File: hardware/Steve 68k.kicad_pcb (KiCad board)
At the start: 2 copper layers, 99 x 98.9 mm, 43 parts, among them IC1 MC68008FN8, J1 Power, J2 I2C, J3 Debug, J4 ICSP, J5 Serial 1, SW1 Reset, U1 74HC04, U2 74HC32, U3 74HC138, U4 74HC257, U5 AS6C4008-55PCN, U6 28C256, U7 ATmega1284P-P, U8 Max705, X1 8Mhz

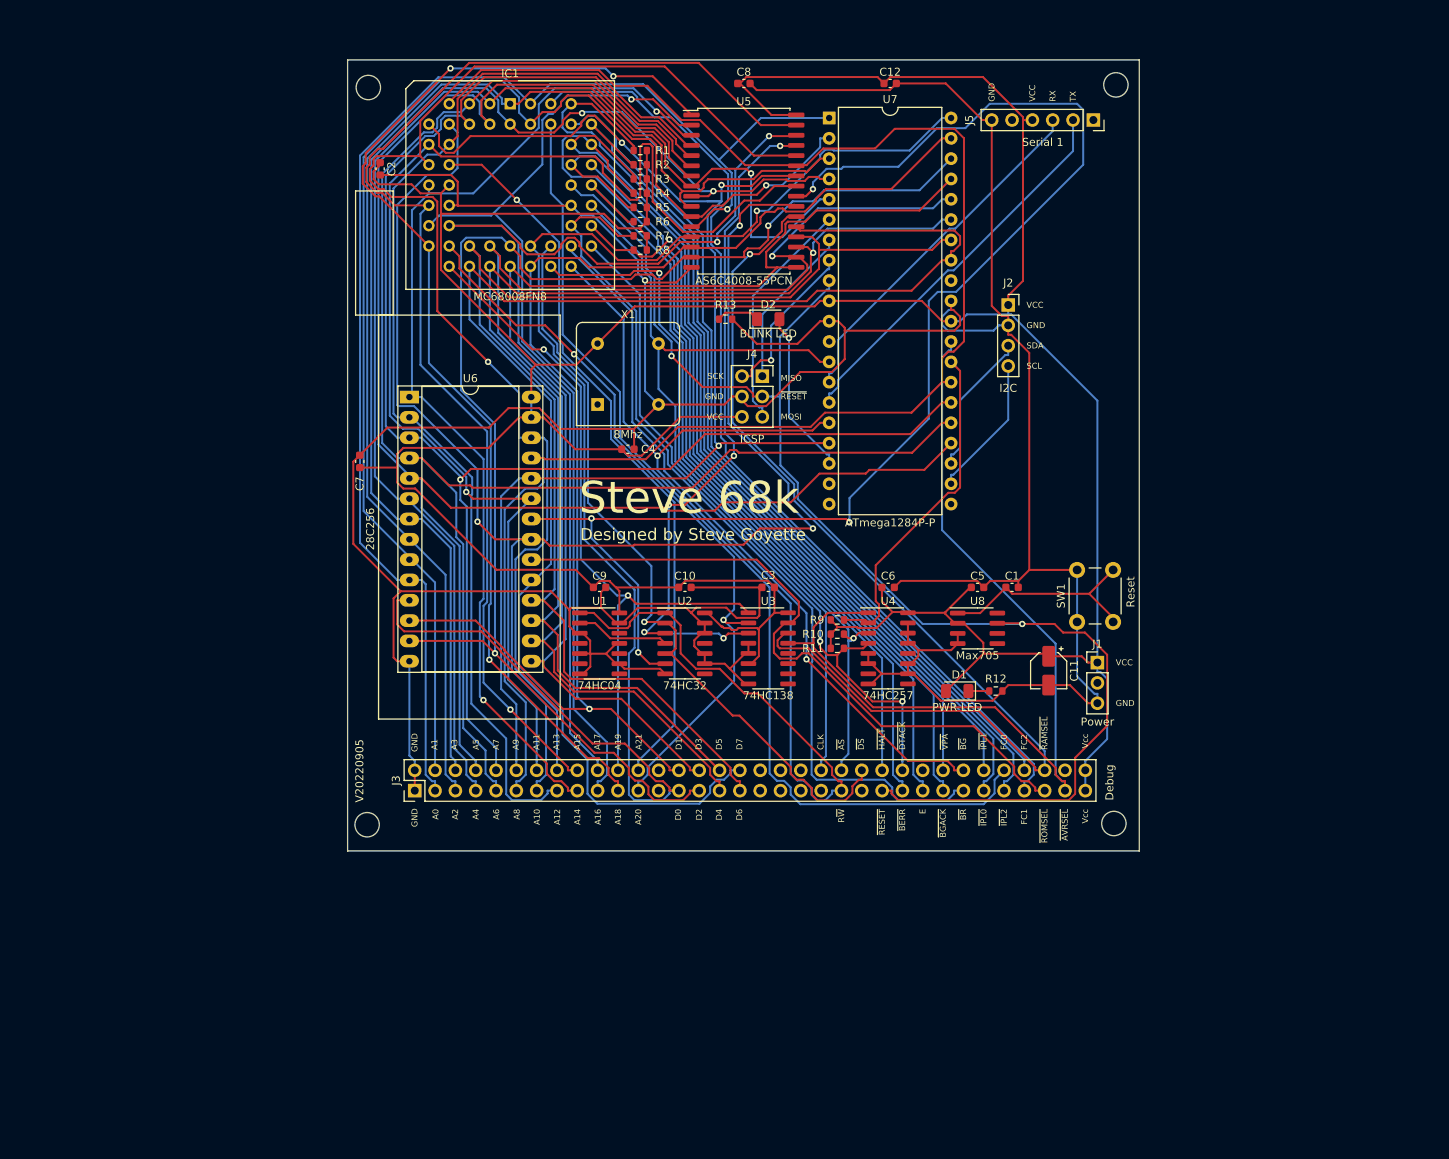
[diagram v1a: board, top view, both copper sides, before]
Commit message: V20221121
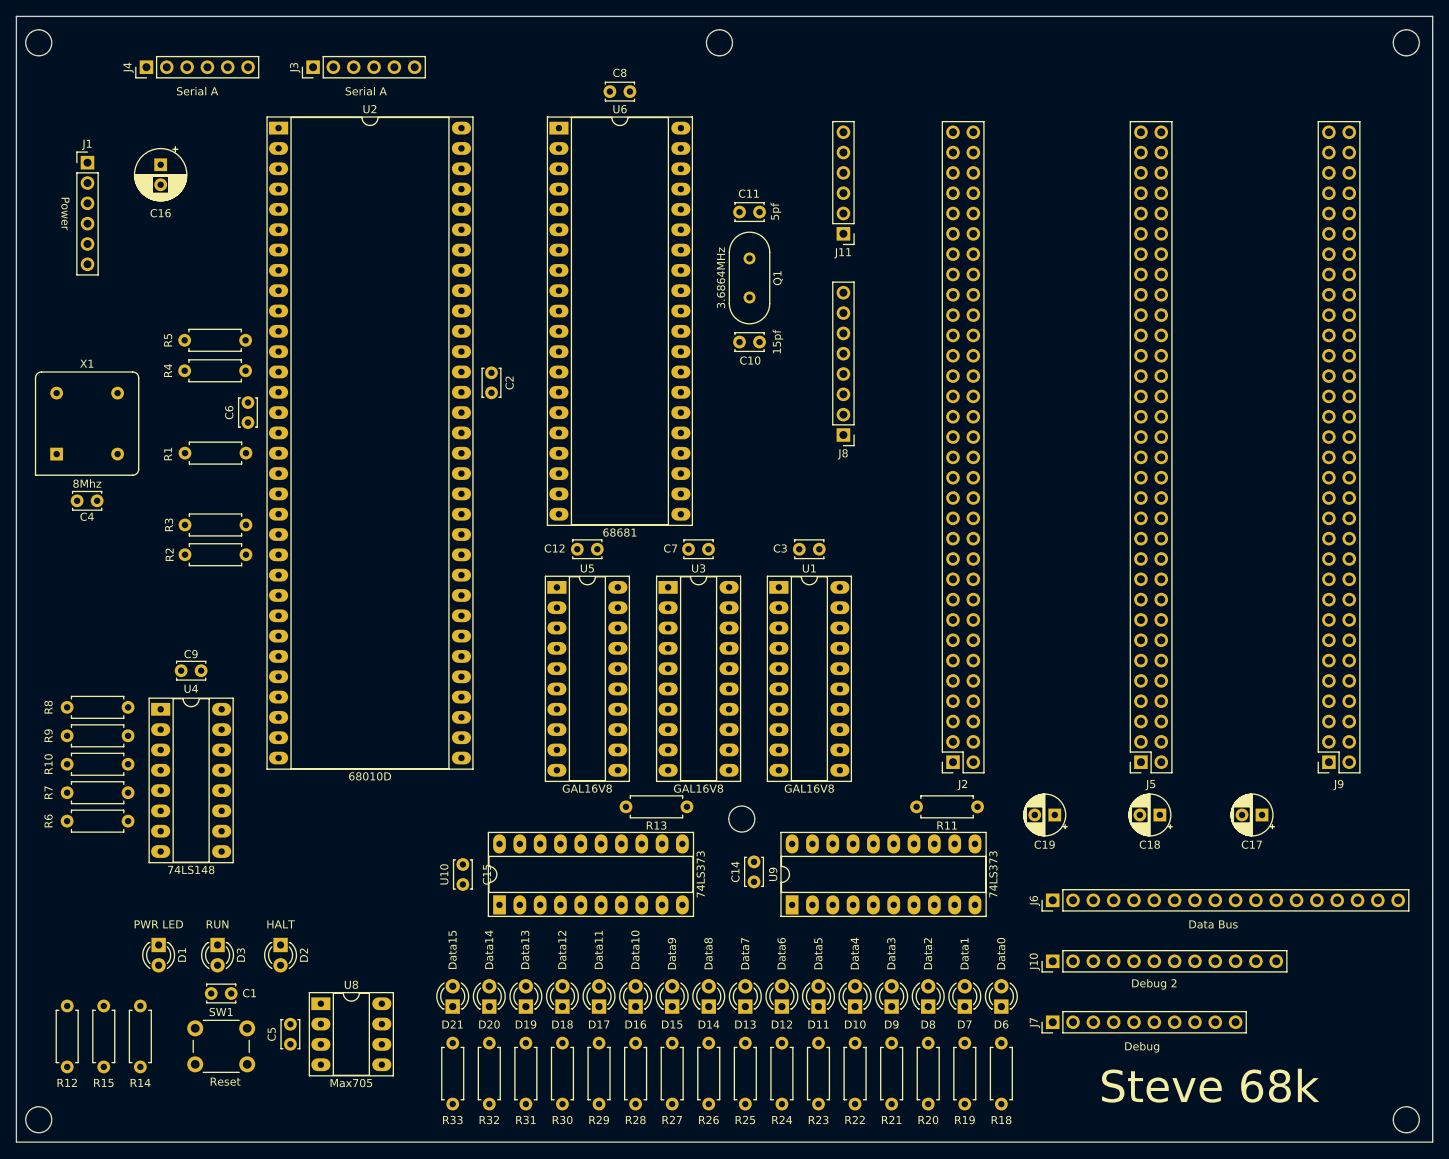
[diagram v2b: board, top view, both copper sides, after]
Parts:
- removed IC1: MC68008FN8, Package_LCC:PLCC-52_THT-Socket
- removed U7: ATmega1284P-P, Package_DIP:DIP-40_W15.24mm
- added C14: .1uF, Capacitor_THT:C_Disc_D3.4mm_W2.1mm_P2.50mm, F.Cu at (114.6, 136.7)
- added C15: .1uF, Capacitor_THT:C_Disc_D3.4mm_W2.1mm_P2.50mm, F.Cu at (78.2, 137.0)
- added C16: 470uF, Capacitor_THT:CP_Radial_D6.3mm_P2.50mm, F.Cu at (40.4, 49.5)
- added C17: 100uF, Capacitor_THT:CP_Radial_D5.0mm_P2.50mm, F.Cu at (178.1, 130.8)
- added C18: 100uF, Capacitor_THT:CP_Radial_D5.0mm_P2.50mm, F.Cu at (165.3, 130.8)
- added C19: 100uF, Capacitor_THT:CP_Radial_D5.0mm_P2.50mm, F.Cu at (152.1, 130.8)
- added D10: Data4, LED_THT:LED_D3.0mm_Clear, F.Cu at (127.2, 154.8)
- added D11: Data5, LED_THT:LED_D3.0mm_Clear, F.Cu at (122.6, 154.8)
- added D12: Data6, LED_THT:LED_D3.0mm_Clear, F.Cu at (118.0, 154.8)
- added D13: Data7, LED_THT:LED_D3.0mm_Clear, F.Cu at (113.5, 154.8)
- added D14: Data8, LED_THT:LED_D3.0mm_Clear, F.Cu at (108.9, 154.8)
- added D15: Data9, LED_THT:LED_D3.0mm_Clear, F.Cu at (104.3, 154.8)
- added D16: Data10, LED_THT:LED_D3.0mm_Clear, F.Cu at (99.8, 154.8)
- added D17: Data11, LED_THT:LED_D3.0mm_Clear, F.Cu at (95.2, 154.8)
- added D18: Data12, LED_THT:LED_D3.0mm_Clear, F.Cu at (90.6, 154.8)
- added D19: Data13, LED_THT:LED_D3.0mm_Clear, F.Cu at (86.0, 154.8)
- added D20: Data14, LED_THT:LED_D3.0mm_Clear, F.Cu at (81.5, 154.8)
- added D21: Data15, LED_THT:LED_D3.0mm_Clear, F.Cu at (76.9, 154.8)
- added D3: RUN, LED_THT:LED_D3.0mm_Clear, F.Cu at (47.5, 147.1)
- added D6: Data0, LED_THT:LED_D3.0mm_Clear, F.Cu at (145.5, 154.8)
- added D7: Data1, LED_THT:LED_D3.0mm_Clear, F.Cu at (140.9, 154.8)
- added D8: Data2, LED_THT:LED_D3.0mm_Clear, F.Cu at (136.3, 154.8)
- added D9: Data3, LED_THT:LED_D3.0mm_Clear, F.Cu at (131.8, 154.8)
- added J10: Debug 2, Connector_PinHeader_2.54mm:PinHeader_1x12_P2.54mm_Vertical, F.Cu at (151.9, 149.1)
- added J11: Duart IP, Connector_PinHeader_2.54mm:PinHeader_1x06_P2.54mm_Vertical, F.Cu at (125.7, 58.2)
- added J6: Data Bus, Connector_PinHeader_2.54mm:PinHeader_1x18_P2.54mm_Vertical, F.Cu at (151.9, 141.5)
- added J7: Debug, Connector_PinHeader_2.54mm:PinHeader_1x10_P2.54mm_Vertical, F.Cu at (151.9, 156.7)
- added J8: Duart OP, Connector_PinHeader_2.54mm:PinHeader_1x08_P2.54mm_Vertical, F.Cu at (125.7, 83.3)
- added J9: Conn_02x32_Odd_Even, Connector_PinSocket_2.54mm:PinSocket_2x32_P2.54mm_Vertical, F.Cu at (186.4, 124.2)
- added Q1: 3.6864MHz, Crystal:Crystal_HC49-4H_Vertical, F.Cu at (114.0, 61.2)
- added R14: 470, Resistor_THT:R_Axial_DIN0207_L6.3mm_D2.5mm_P7.62mm_Horizontal, F.Cu at (37.8, 162.3)
- added R15: 470, Resistor_THT:R_Axial_DIN0207_L6.3mm_D2.5mm_P7.62mm_Horizontal, F.Cu at (33.3, 162.3)
- added R18: 470, Resistor_THT:R_Axial_DIN0207_L6.3mm_D2.5mm_P7.62mm_Horizontal, F.Cu at (145.5, 166.9)
- added R19: 470, Resistor_THT:R_Axial_DIN0207_L6.3mm_D2.5mm_P7.62mm_Horizontal, F.Cu at (140.9, 166.9)
- added R20: 470, Resistor_THT:R_Axial_DIN0207_L6.3mm_D2.5mm_P7.62mm_Horizontal, F.Cu at (136.3, 166.9)
- added R21: 470, Resistor_THT:R_Axial_DIN0207_L6.3mm_D2.5mm_P7.62mm_Horizontal, F.Cu at (131.8, 166.9)
- added R22: 470, Resistor_THT:R_Axial_DIN0207_L6.3mm_D2.5mm_P7.62mm_Horizontal, F.Cu at (127.2, 166.9)
- added R23: 470, Resistor_THT:R_Axial_DIN0207_L6.3mm_D2.5mm_P7.62mm_Horizontal, F.Cu at (122.6, 166.9)
- added R24: 470, Resistor_THT:R_Axial_DIN0207_L6.3mm_D2.5mm_P7.62mm_Horizontal, F.Cu at (118.0, 166.9)
- added R25: 470, Resistor_THT:R_Axial_DIN0207_L6.3mm_D2.5mm_P7.62mm_Horizontal, F.Cu at (113.5, 166.9)
- added R26: 470, Resistor_THT:R_Axial_DIN0207_L6.3mm_D2.5mm_P7.62mm_Horizontal, F.Cu at (108.9, 166.9)
- added R27: 470, Resistor_THT:R_Axial_DIN0207_L6.3mm_D2.5mm_P7.62mm_Horizontal, F.Cu at (104.3, 166.9)
- added R28: 470, Resistor_THT:R_Axial_DIN0207_L6.3mm_D2.5mm_P7.62mm_Horizontal, F.Cu at (99.8, 166.9)
- added R29: 470, Resistor_THT:R_Axial_DIN0207_L6.3mm_D2.5mm_P7.62mm_Horizontal, F.Cu at (95.2, 166.9)
- added R30: 470, Resistor_THT:R_Axial_DIN0207_L6.3mm_D2.5mm_P7.62mm_Horizontal, F.Cu at (90.6, 166.9)
- added R31: 470, Resistor_THT:R_Axial_DIN0207_L6.3mm_D2.5mm_P7.62mm_Horizontal, F.Cu at (86.0, 166.9)
- added R32: 470, Resistor_THT:R_Axial_DIN0207_L6.3mm_D2.5mm_P7.62mm_Horizontal, F.Cu at (81.5, 166.9)
- added R33: 470, Resistor_THT:R_Axial_DIN0207_L6.3mm_D2.5mm_P7.62mm_Horizontal, F.Cu at (76.9, 166.9)
- added U10: 74LS373, Package_DIP:DIP-20_W7.62mm_Socket_LongPads, F.Cu at (82.7, 142.1)
- added U9: 74LS373, Package_DIP:DIP-20_W7.62mm_Socket_LongPads, F.Cu at (119.3, 142.1)
- C1, C12, C2, C3, C4, C5, C6, C7, C8, C9: footprint Capacitor_SMD:C_0603_1608Metric -> Capacitor_THT:C_Disc_D3.4mm_W2.1mm_P2.50mm
- C10: value .1uF -> 15pf; footprint Capacitor_SMD:C_0603_1608Metric -> Capacitor_THT:C_Disc_D3.4mm_W2.1mm_P2.50mm
- C11: value 100uF -> 5pf; footprint Capacitor_SMD:CP_Elec_4x5.4 -> Capacitor_THT:C_Disc_D3.4mm_W2.1mm_P2.50mm
- D1: footprint LED_SMD:LED_1206_3216Metric -> LED_THT:LED_D3.0mm_Clear
- D2: value BLINK LED -> HALT; footprint LED_SMD:LED_1206_3216Metric -> LED_THT:LED_D3.0mm_Clear
- J1: footprint Connector_PinHeader_2.54mm:PinHeader_1x03_P2.54mm_Vertical -> Connector_PinHeader_2.54mm:PinHeader_1x06_P2.54mm_Vertical
- J2: value I2C -> Conn_02x32_Odd_Even; footprint Connector_PinSocket_2.54mm:PinSocket_1x04_P2.54mm_Vertical -> Connector_PinSocket_2.54mm:PinSocket_2x32_P2.54mm_Vertical
- J3: value Debug -> Serial A; footprint Connector_PinHeader_2.54mm:PinHeader_2x34_P2.54mm_Vertical -> Connector_PinHeader_2.54mm:PinHeader_1x06_P2.54mm_Vertical
- J4: value ICSP -> Serial A; footprint Connector_PinSocket_2.54mm:PinSocket_2x03_P2.54mm_Vertical -> Connector_PinHeader_2.54mm:PinHeader_1x06_P2.54mm_Vertical
- J5: value Serial 1 -> Conn_02x32_Odd_Even; footprint Connector_PinSocket_2.54mm:PinSocket_1x06_P2.54mm_Vertical -> Connector_PinSocket_2.54mm:PinSocket_2x32_P2.54mm_Vertical
- R1: value 10k -> Rk7; footprint Resistor_SMD:R_0603_1608Metric -> Resistor_THT:R_Axial_DIN0207_L6.3mm_D2.5mm_P7.62mm_Horizontal
- R10, R2, R3, R4, R5, R6, R7, R8, R9: value 10k -> 4K7; footprint Resistor_SMD:R_0603_1608Metric -> Resistor_THT:R_Axial_DIN0207_L6.3mm_D2.5mm_P7.62mm_Horizontal
- R11: value 10k -> 4k7; footprint Resistor_SMD:R_0603_1608Metric -> Resistor_THT:R_Axial_DIN0207_L6.3mm_D2.5mm_P7.62mm_Horizontal
- R12: value 220 -> 470; footprint Resistor_SMD:R_0603_1608Metric -> Resistor_THT:R_Axial_DIN0207_L6.3mm_D2.5mm_P7.62mm_Horizontal
- R13: value 220 -> 4k7; footprint Resistor_SMD:R_0603_1608Metric -> Resistor_THT:R_Axial_DIN0207_L6.3mm_D2.5mm_P7.62mm_Horizontal
- U1: value 74HC04 -> GAL16V8; footprint Package_SO:SOIC-14_3.9x8.7mm_P1.27mm -> Package_DIP:DIP-20_W7.62mm_Socket_LongPads
- U2: value 74HC32 -> 68010D; footprint Package_SO:SOIC-14_3.9x8.7mm_P1.27mm -> Package_DIP:DIP-64_W22.86mm_Socket_LongPads
- U3: value 74HC138 -> GAL16V8; footprint Package_SO:SOIC-16_3.9x9.9mm_P1.27mm -> Package_DIP:DIP-20_W7.62mm_Socket_LongPads
- U4: value 74HC257 -> 74LS148; footprint Package_SO:SOIC-16_3.9x9.9mm_P1.27mm -> Package_DIP:DIP-16_W7.62mm_Socket_LongPads
- U5: value AS6C4008-55PCN -> GAL16V8; footprint Package_SO:SSOP-32_11.305x20.495mm_P1.27mm -> Package_DIP:DIP-20_W7.62mm_Socket_LongPads
- U6: value 28C256 -> 68681; footprint Package_DIP:DIP-28_W15.24mm_Socket_LongPads -> Package_DIP:DIP-40_W15.24mm_Socket_LongPads
- U8: footprint Package_SO:SOIC-8_3.9x4.9mm_P1.27mm -> Package_DIP:DIP-8_W7.62mm_Socket_LongPads
- moved J1 140.9 mm to (31.2, 49.3)
- moved R12 125.2 mm to (28.7, 162.3), turned to 90 degrees
- moved SW1 121.4 mm to (44.7, 157.5), turned to 0 degrees
- moved C1 110.0 mm to (49.2, 153.1), turned to 180 degrees
- moved D1 104.7 mm to (40.1, 147.1), turned to -90 degrees
- moved R6 103.7 mm to (28.7, 131.6), turned to 0 degrees
- moved C5 103.1 mm to (56.6, 159.5), turned to 90 degrees
- moved R7 99.9 mm to (28.7, 128.0), turned to 0 degrees
- moved D2 99.2 mm to (55.4, 147.1), turned to -90 degrees
- moved R10 97.6 mm to (28.7, 124.5)
- moved R9 97.4 mm to (28.7, 120.9)
- moved U8 94.5 mm to (60.4, 154.4)
- moved R8 91.6 mm to (28.7, 117.4), turned to 0 degrees
- moved J3 91.3 mm to (59.4, 37.3)
- moved U4 91.3 mm to (40.4, 117.6)
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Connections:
- C10 pad 1: VCC -> Net-(C10-Pad1)
- C11 pad 1: VCC -> Net-(C11-Pad1)
- C2 pad 1: VCC -> GND
- C2 pad 2: GND -> VCC
- C6 pad 1: VCC -> GND
- C6 pad 2: GND -> VCC
- D1 pad 1: Net-(D1-Pad1) -> VCC
- D1 pad 2: VCC -> Net-(D1-Pad2)
- D2 pad 1: Net-(D2-Pad1) -> VCC
- J1 pad 2: unconnected-(J1-Pad2) -> GND
- J1 pad 3: GND -> unconnected-(J1-Pad3)
- J2 pad 1: VCC -> /A1
- J2 pad 2: GND -> VCC
- J2 pad 3: /SDA -> /A2
- J2 pad 4: /SCL -> /CLK
- J3 pad 1: GND -> /CTSA
- J3 pad 2: GND -> /TXDA
- J3 pad 3: /A0 -> /RXDA
- J3 pad 4: /A1 -> unconnected-(J3-Pad4)
- J3 pad 5: /A2 -> /RTSA
- J3 pad 6: /A3 -> GND
- J4 pad 1: /MISO -> /CTSB
- J4 pad 2: /SCK -> /TXDB
- J4 pad 3: /~{RESET} -> /RXDB
- J4 pad 4: GND -> unconnected-(J4-Pad4)
- J4 pad 5: /MOSI -> /RTSB
- J4 pad 6: VCC -> GND
- J5 pad 1: unconnected-(J5-Pad1) -> /A1
- J5 pad 2: /TXD0 -> VCC
- J5 pad 3: /RXD0 -> /A2
- J5 pad 4: VCC -> /CLK
- J5 pad 5: unconnected-(J5-Pad5) -> /A3
- R1 pad 2: /~{IPL0} -> /~{HALT}
- R10 pad 2: /~{AS} -> /~{IRQ6}
- R11 pad 1: VCC -> /STATUSLO
- R11 pad 2: /~{DTACK_CPU} -> VCC
- R12 pad 2: Net-(D1-Pad1) -> Net-(D1-Pad2)
- R13 pad 1: GND -> /STATUSHI
- R13 pad 2: Net-(D2-Pad1) -> VCC
- R2 pad 2: /~{IPL2} -> /~{BERR}
- R3 pad 2: /~{IPL1} -> /~{VPA}
- R4 pad 2: /~{BERR} -> /~{BR}
- R5 pad 2: /~{VPA} -> /~{BGACK}
- R6 pad 2: /~{HALT} -> /~{IRQ2}
- R7 pad 2: /~{BR} -> /~{IRQ3}
- R8 pad 2: /~{BGACK} -> /~{IRQ4}
- R9 pad 2: /~{DTACK_AVR} -> /~{IRQ5}
- U1 pad 1: /R~{W} -> /CLK
- U1 pad 10: unconnected-(U1-Pad10) -> GND
- U1 pad 11: GND -> unconnected-(U1-Pad11)
- U1 pad 13: GND -> unconnected-(U1-Pad13)
- U1 pad 14: VCC -> unconnected-(U1-Pad14)
- U1 pad 2: Net-(U1-Pad2) -> /A1
- U1 pad 3: GND -> /A2
- U1 pad 4: unconnected-(U1-Pad4) -> /A3
- U1 pad 5: GND -> /FC0
- U1 pad 6: unconnected-(U1-Pad6) -> /FC1
- U1 pad 7: GND -> /FC2
- U1 pad 8: unconnected-(U1-Pad8) -> /~{HALT}
- U1 pad 9: GND -> /~{RESET}
- U2 pad 1: /R~{W} -> /D4
- U2 pad 10: GND -> /~{DTACK}
- U2 pad 11: unconnected-(U2-Pad11) -> /~{BG}
- U2 pad 12: GND -> /~{BGACK}
- U2 pad 13: GND -> /~{BR}
- U2 pad 2: /~{DS} -> /D3
- U2 pad 3: /~{RAM_WE} -> /D2
- U2 pad 4: Net-(U1-Pad2) -> /D1
- U2 pad 5: /~{DS} -> /D0
- U2 pad 6: /~{OE} -> /~{AS}
- U2 pad 7: GND -> /~{UDS}
- U2 pad 8: unconnected-(U2-Pad8) -> /~{LDS}
- U2 pad 9: GND -> /R~{W}
- U3 pad 10: unconnected-(U3-Pad10) -> GND
- U3 pad 13: /~{AVRSEL} -> unconnected-(U3-Pad13)
- U3 pad 14: /~{RAMSEL} -> unconnected-(U3-Pad14)
- U3 pad 15: /~{ROMSEL} -> unconnected-(U3-Pad15)
- U3 pad 16: VCC -> unconnected-(U3-Pad16)
- U3 pad 4: GND -> /A22
- U3 pad 5: GND -> /A23
- U3 pad 6: VCC -> /~{AS}
- U3 pad 7: unconnected-(U3-Pad7) -> /~{UDS}
- U3 pad 8: GND -> /~{LDS}
- U3 pad 9: unconnected-(U3-Pad9) -> /~{RESET}
- U4 pad 1: /~{AVRSEL} -> /~{IRQ4}
- U4 pad 11: GND -> VCC
- U4 pad 12: unconnected-(U4-Pad12) -> /~{IRQ2}
- U4 pad 13: GND -> /~{IRQ3}
- U4 pad 14: GND -> unconnected-(U4-Pad14)
- U4 pad 15: GND -> unconnected-(U4-Pad15)
- U4 pad 2: /~{DTACK_AVR} -> /~{IRQ5}
- U4 pad 3: /~{AS} -> /~{IRQ6}
- U4 pad 4: /~{DTACK_CPU} -> VCC
- U4 pad 6: GND -> /~{IPL2}
- U4 pad 7: unconnected-(U4-Pad7) -> /~{IPL1}
- U4 pad 9: unconnected-(U4-Pad9) -> /~{IPL0}
- U5 pad 1: /A18 -> /~{UDS}
- U5 pad 10: /A2 -> GND
- U5 pad 11: /A1 -> unconnected-(U5-Pad11)
- U5 pad 12: /A0 -> unconnected-(U5-Pad12)
- U5 pad 13: /D0 -> unconnected-(U5-Pad13)
- U5 pad 14: /D1 -> unconnected-(U5-Pad14)
- U5 pad 15: /D2 -> unconnected-(U5-Pad15)
- U5 pad 16: GND -> /STATUSHI
- U5 pad 17: /D3 -> /STATUSLO
- U5 pad 18: /D4 -> /~{DTACK}
- U5 pad 19: /D5 -> /~{UARTSEL}
- U5 pad 2: /A16 -> /~{LDS}
- U5 pad 20: /D6 -> VCC
- U5 pad 3: /A14 -> /R~{W}
- U5 pad 4: /A12 -> /A18
- U5 pad 5: /A7 -> /A17
- U5 pad 6: /A6 -> /A16
- U5 pad 7: /A5 -> /A15
- U5 pad 8: /A4 -> /A14
- U5 pad 9: /A3 -> /~{IOSEL}
- U6 pad 1: /A14 -> /A1
- U6 pad 10: /A0 -> /RXDB
- U6 pad 11: /D0 -> /TXDB
- U6 pad 12: /D1 -> /RTSB
- U6 pad 13: /D2 -> /OP3
- U6 pad 14: GND -> /OP5
- U6 pad 15: /D3 -> /OP7
- U6 pad 16: /D4 -> /D1
- U6 pad 17: /D5 -> /D3
- U6 pad 18: /D6 -> /D5
- U6 pad 2: /A12 -> /IP3
- U6 pad 20: /~{ROMSEL} -> GND
- U6 pad 21: /A10 -> /~{IRQ2}
- U6 pad 22: /~{OE} -> /D6
- U6 pad 23: /A11 -> /D4
- U6 pad 24: /A9 -> /D2
- U6 pad 25: /A8 -> /D0
- U6 pad 26: /A13 -> /OP6
- U6 pad 27: VCC -> /OP4
- U6 pad 28: VCC -> /OP2
- U6 pad 3: /A7 -> /A2
- U6 pad 4: /A6 -> /CTSB
- U6 pad 5: /A5 -> /A3
- U6 pad 7: /A3 -> /CTSA
- U6 pad 8: /A2 -> /R~{W}
- U6 pad 9: /A1 -> /~{DTACK}
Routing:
- net GND: track 528.6 -> 0.00 mm, vias 1 -> 0
- net VCC: track 480.0 -> 0.00 mm
- net /A5: track 211.0 -> 0.00 mm
- net /A8: track 209.9 -> 0.00 mm
- net /A6: track 207.1 -> 0.00 mm
- net /A7: track 199.6 -> 0.00 mm, vias 1 -> 0
- net /D0: track 193.7 -> 0.00 mm, vias 1 -> 0
- net /A10: track 192.1 -> 0.00 mm, vias 3 -> 0
- net /D7: track 186.5 -> 0.00 mm
- net /D2: track 172.0 -> 0.00 mm, vias 2 -> 0
- net /A9: track 169.6 -> 0.00 mm, vias 3 -> 0
- net /~{OE}: track 169.5 -> 0.00 mm, vias 4 -> 0
- net /A0: track 168.9 -> 0.00 mm, vias 1 -> 0
- net /~{RESET}: track 168.4 -> 0.00 mm, vias 2 -> 0
- net /A4: track 164.4 -> 0.00 mm, vias 1 -> 0
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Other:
- board size 99 x 98.9 mm -> 177 x 140.7 mm
- board text removed: "A0"
- board text removed: "A1"
- board text removed: "A10"
- board text removed: "A11"
- board text removed: "A12"
- board text removed: "A13"
- board text removed: "A14"
- board text removed: "A15"
- board text removed: "A16"
- board text removed: "A17"
- board text removed: "A18"
- board text removed: "A19"
- board text removed: "A2"
- board text removed: "A20"
- board text removed: "A21"
- board text removed: "A3"
- board text removed: "A4"
- board text removed: "A5"
- board text removed: "A6"
- board text removed: "A7"
- board text removed: "A8"
- board text removed: "A9"
- board text removed: "CLK"
- board text removed: "D0"
- board text removed: "D1"
- board text removed: "D2"
- board text removed: "D3"
- board text removed: "D4"
- board text removed: "D5"
- board text removed: "D6"
- board text removed: "D7"
- board text removed: "Designed by Steve Goyette"
- board text removed: "E"
- board text removed: "FC0"
- board text removed: "FC1"
- board text removed: "FC2"
- board text removed: "GND"
- board text removed: "MISO"
- board text removed: "MOSI"
- board text removed: "RX"
- board text removed: "R~{W}"
- board text removed: "SCK"
- board text removed: "SCL"
- board text removed: "SDA"
- board text removed: "TX"
- board text removed: "V20220905"
- board text removed: "VCC"
- board text removed: "Vcc"
- board text removed: "~{AS}"
- board text removed: "~{AVRSEL}"
- board text removed: "~{BERR}"
- board text removed: "~{BGACK}"
- board text removed: "~{BG}"
- board text removed: "~{BR}"
- board text removed: "~{DS}"
- board text removed: "~{DTACK}"
- board text removed: "~{HALT}"
- board text removed: "~{IPL0}"
- board text removed: "~{IPL1}"
- board text removed: "~{IPL2}"
- board text removed: "~{RAMSEL}"
- board text removed: "~{RESET}"
- board text removed: "~{ROMSEL}"
- board text removed: "~{VPA}"
